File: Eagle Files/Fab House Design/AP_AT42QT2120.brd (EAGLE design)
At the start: 20 x 40 mm, 12 parts, among them U1 AT42QT2120

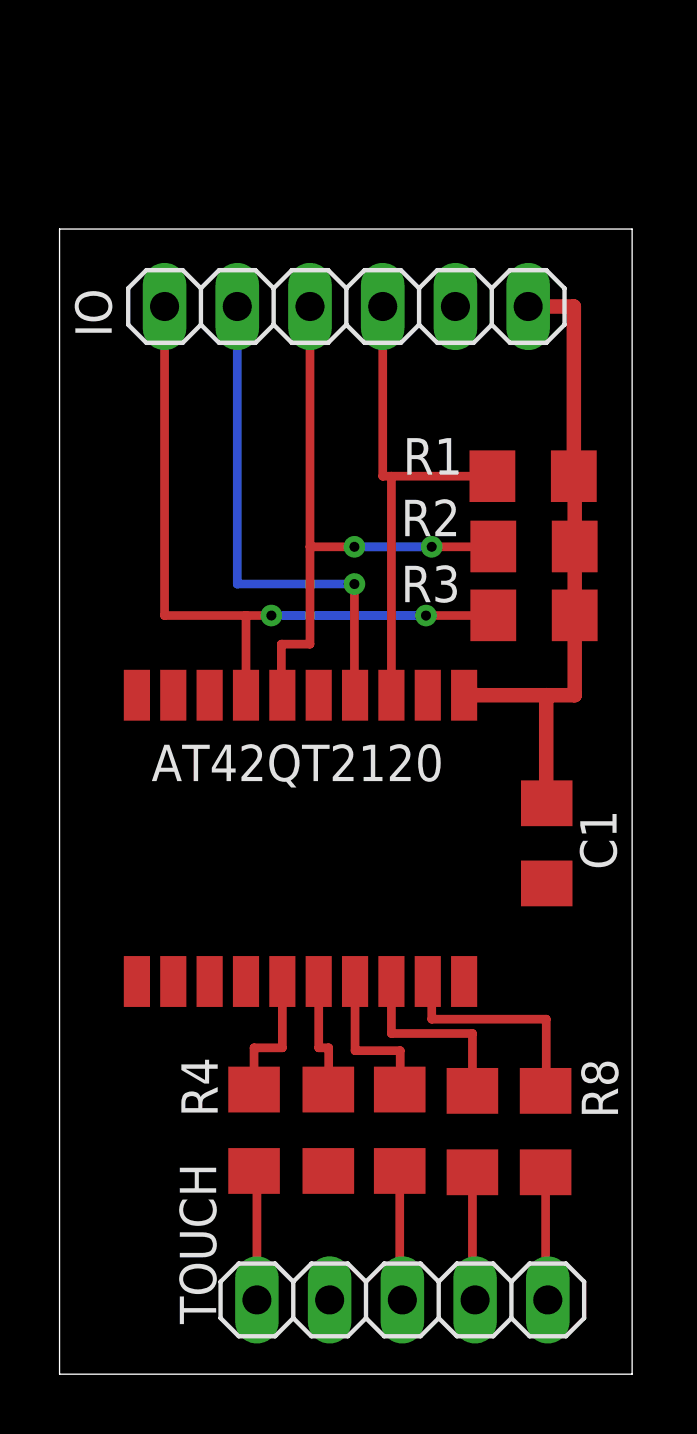
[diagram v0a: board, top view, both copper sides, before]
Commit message: finals
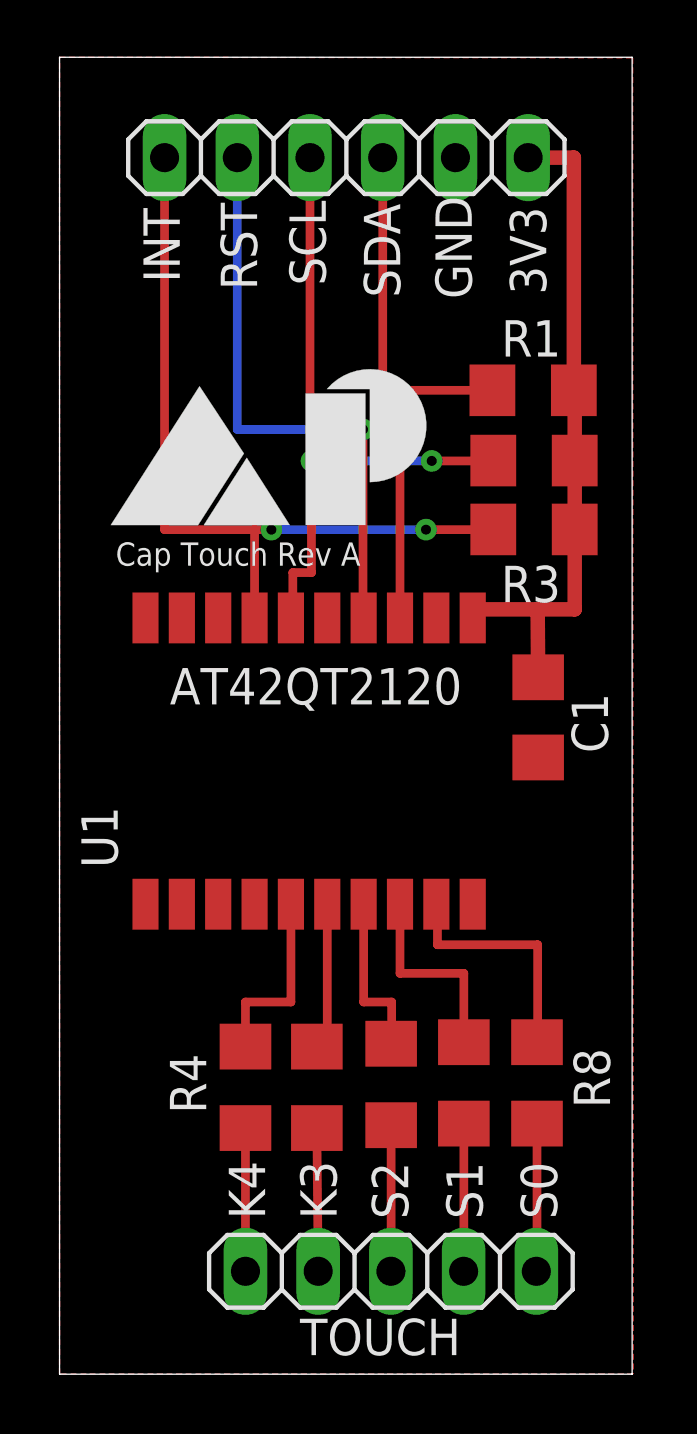
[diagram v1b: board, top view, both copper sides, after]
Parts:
- moved IO 5.20 mm to (10.0, 42.5)
- moved C1 4.41 mm to (16.7, 22.9)
- moved R1 3.00 mm to (16.5, 34.4)
- moved R2 3.00 mm to (16.6, 31.9)
- moved R3 3.00 mm to (16.6, 29.5)
- moved U1 2.72 mm to (3.00, 16.4)
- moved R7 1.73 mm to (14.1, 10.2)
- moved R8 1.73 mm to (16.7, 10.2)
- moved R6 1.63 mm to (11.6, 10.1)
- moved R5 1.55 mm to (8.99, 10.0)
- moved R4 1.53 mm to (6.49, 10.0)
- moved TOUCH 1.08 mm to (11.6, 3.59)
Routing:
- net N$2: track 0.00 -> 5.00 mm
- net N$1: track 17.7 -> 20.5 mm
- net N$26: track 25.1 -> 27.6 mm
- net N$27: track 17.4 -> 19.9 mm
- net N$25: track 21.3 -> 23.4 mm
- net N$5: track 4.76 -> 6.56 mm
- net N$6: track 4.13 -> 5.40 mm
- net N$10: track 4.53 -> 5.17 mm
- net N$11: track 4.55 -> 5.17 mm
- net N$12: track 4.60 -> 5.11 mm
- added copper zone on layer 1, net GND
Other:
- board size 20 x 40 mm -> 20 x 46 mm
- board text added: "3V3"
- board text added: "Cap Touch Rev A"
- board text added: "GND"
- board text added: "INT"
- board text added: "K3"
- board text added: "K4"
- board text added: "RST"
- board text added: "S0"
- board text added: "S1"
- board text added: "S2"
- board text added: "SCL"
- board text added: "SDA"
